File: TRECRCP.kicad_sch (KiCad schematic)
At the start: 16 parts, among them SW1 Dispatch2, SW4 Restart, SW5 Dispatch1, SW6 3 position key switch, SW7 Maintanance rotary switch, SW8 Stop

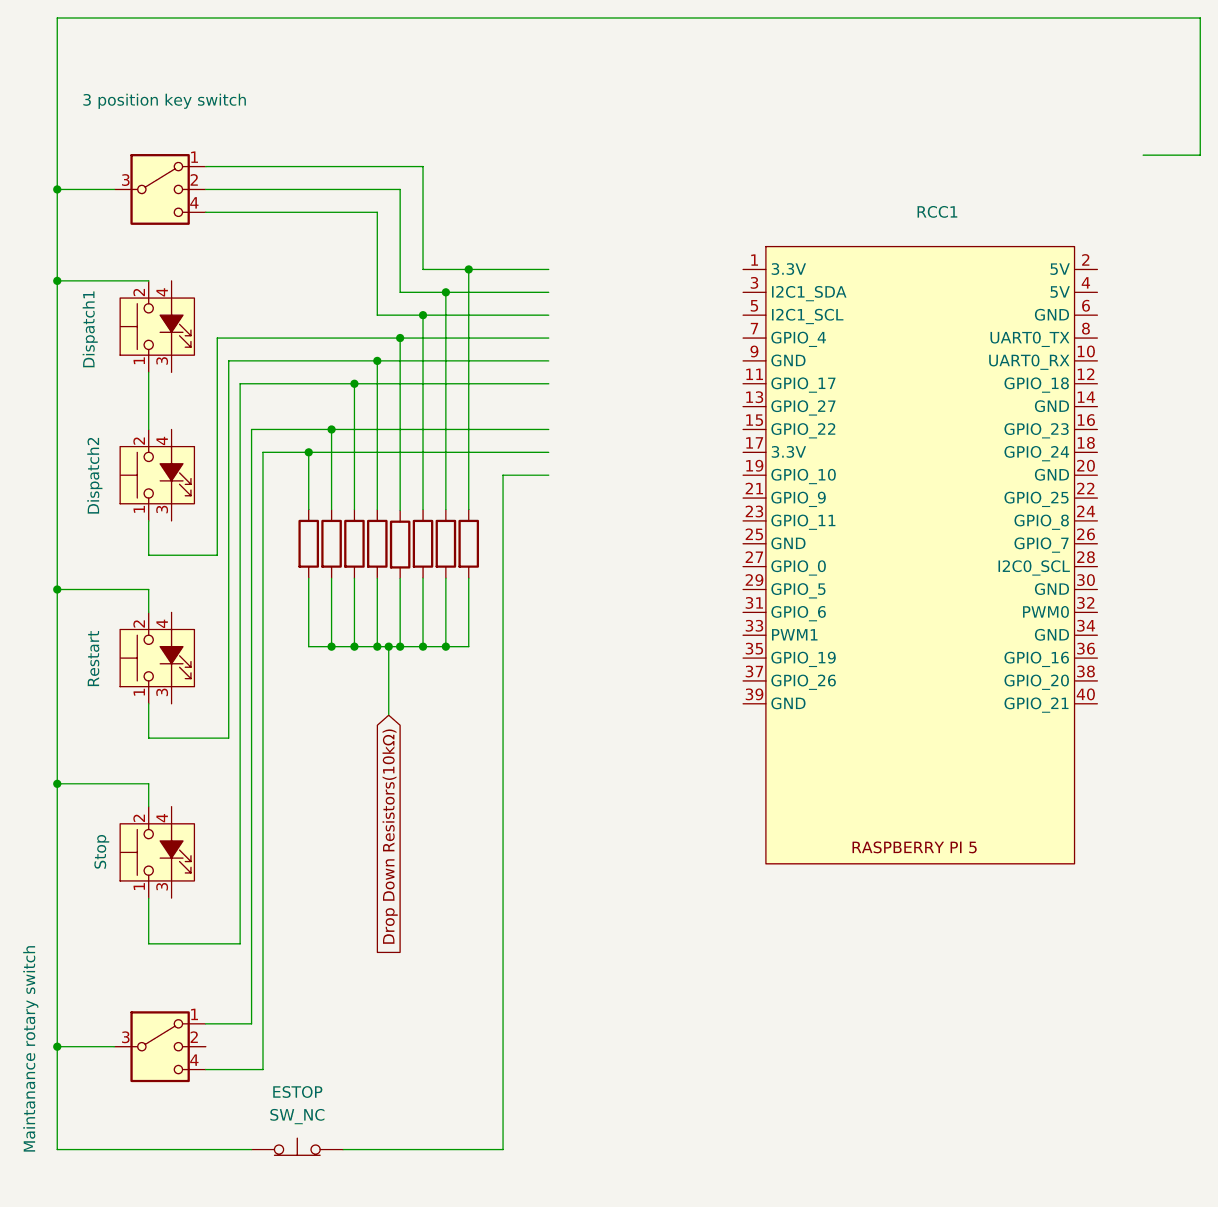
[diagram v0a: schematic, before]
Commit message: Cleanup RCC
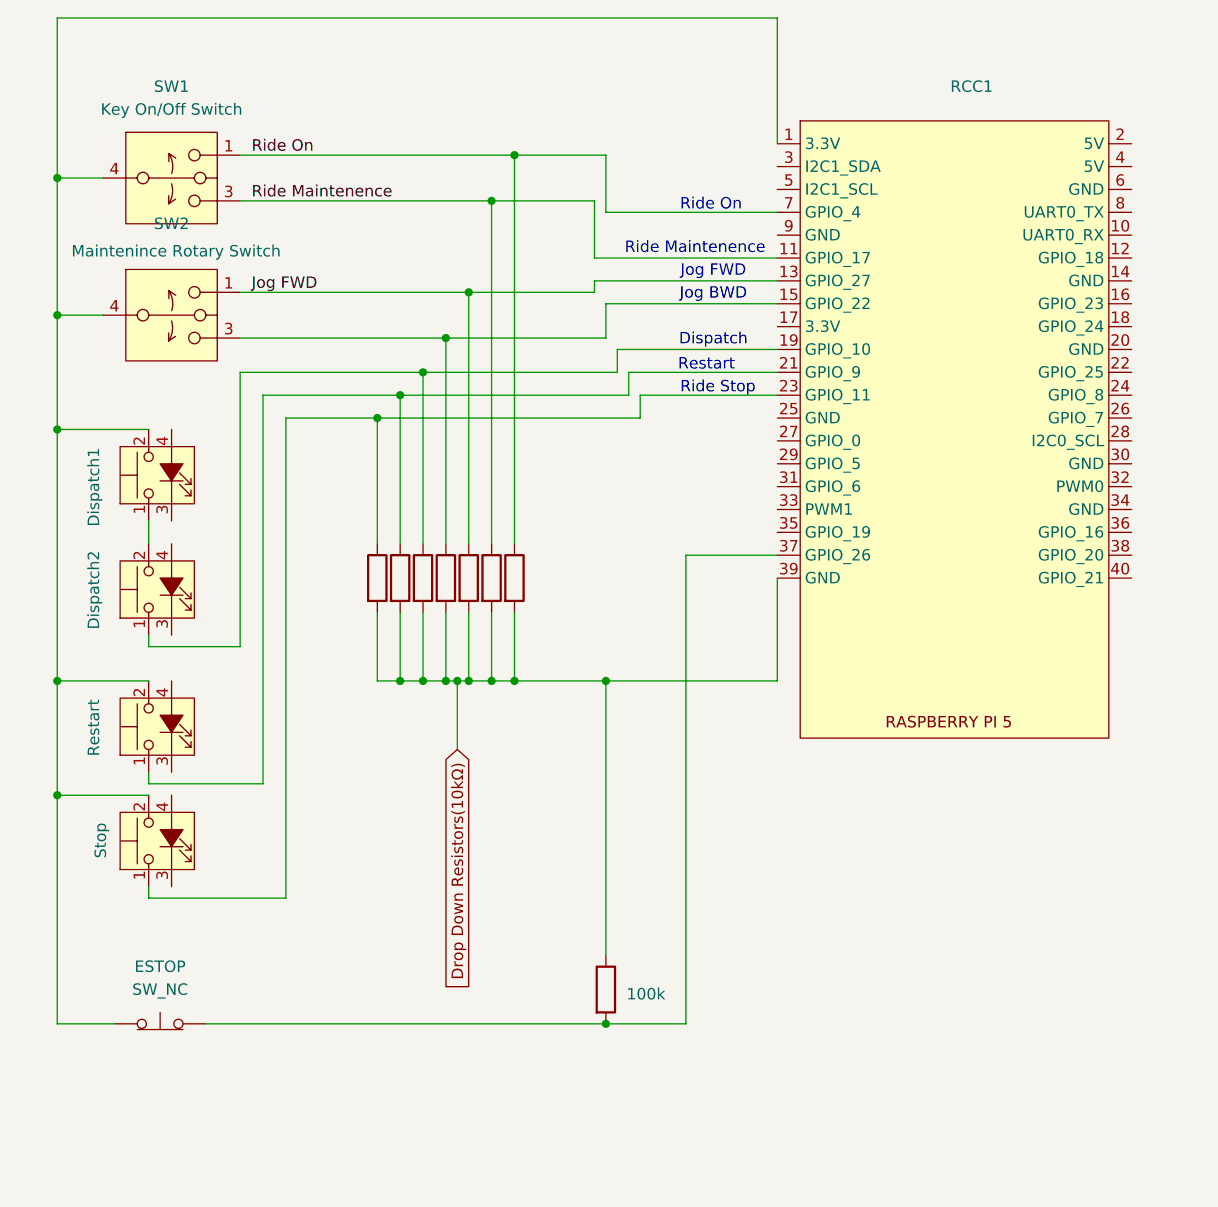
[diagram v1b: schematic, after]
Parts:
- removed SW6: 3 position key switch, symbol Switch:SW_DP3T
- removed SW7: Maintanance rotary switch, symbol Switch:SW_DP3T
- added SW1: Key On/Off Switch, symbol Switch:SW_Rotary_1x3_MP
- added SW2: Maintenince Rotary Switch, symbol Switch:SW_Rotary_1x3_MP
- R8: value R -> 100k
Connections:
- net Drop Down Resistors(10kΩ): now also R8.1, RCC1.39 (GND); no longer R8.2
- net Ride On: now reaches R7.1
- net Ride On: now also RCC1.7 (GPIO_4), SW1.1
- net Ride Maintenence: now reaches R6.1
- net Ride Maintenence: now also RCC1.11 (GPIO_17), SW1.3
- net at SW8.1: now also R1.1, RCC1.23 (GPIO_11); no longer R3.1
- net at ESTOP.1 (A), SW4.2, SW5.2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: now also RCC1.1 (3.3V), SW1.4, SW2.4
- net at ESTOP.2 (B): now also R8.2, RCC1.37 (GPIO_26)
- net at SW1.1: now also R3.1, RCC1.19 (GPIO_10); no longer R5.1
- net at SW4.1: now also R2.1, RCC1.21 (GPIO_9); no longer R4.1
- net Jog FWD: now reaches RCC1.13 (GPIO_27)
- net Jog FWD: now also R5.1, SW2.1
- net at RCC1.15 (GPIO_22): now also R4.1, SW2.3
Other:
- note added: "Dispatch"
- note added: "Jog BWD"
- note added: "Jog FWD"
- note added: "Restart"
- note added: "Ride Maintenence"
- note added: "Ride On"
- note added: "Ride Stop"
- moved on the sheet: ESTOP, RCC1
